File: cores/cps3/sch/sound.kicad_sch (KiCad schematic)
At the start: 68 parts, among them J1 AudioJack2, J2 AudioJack2, Q8 ZR

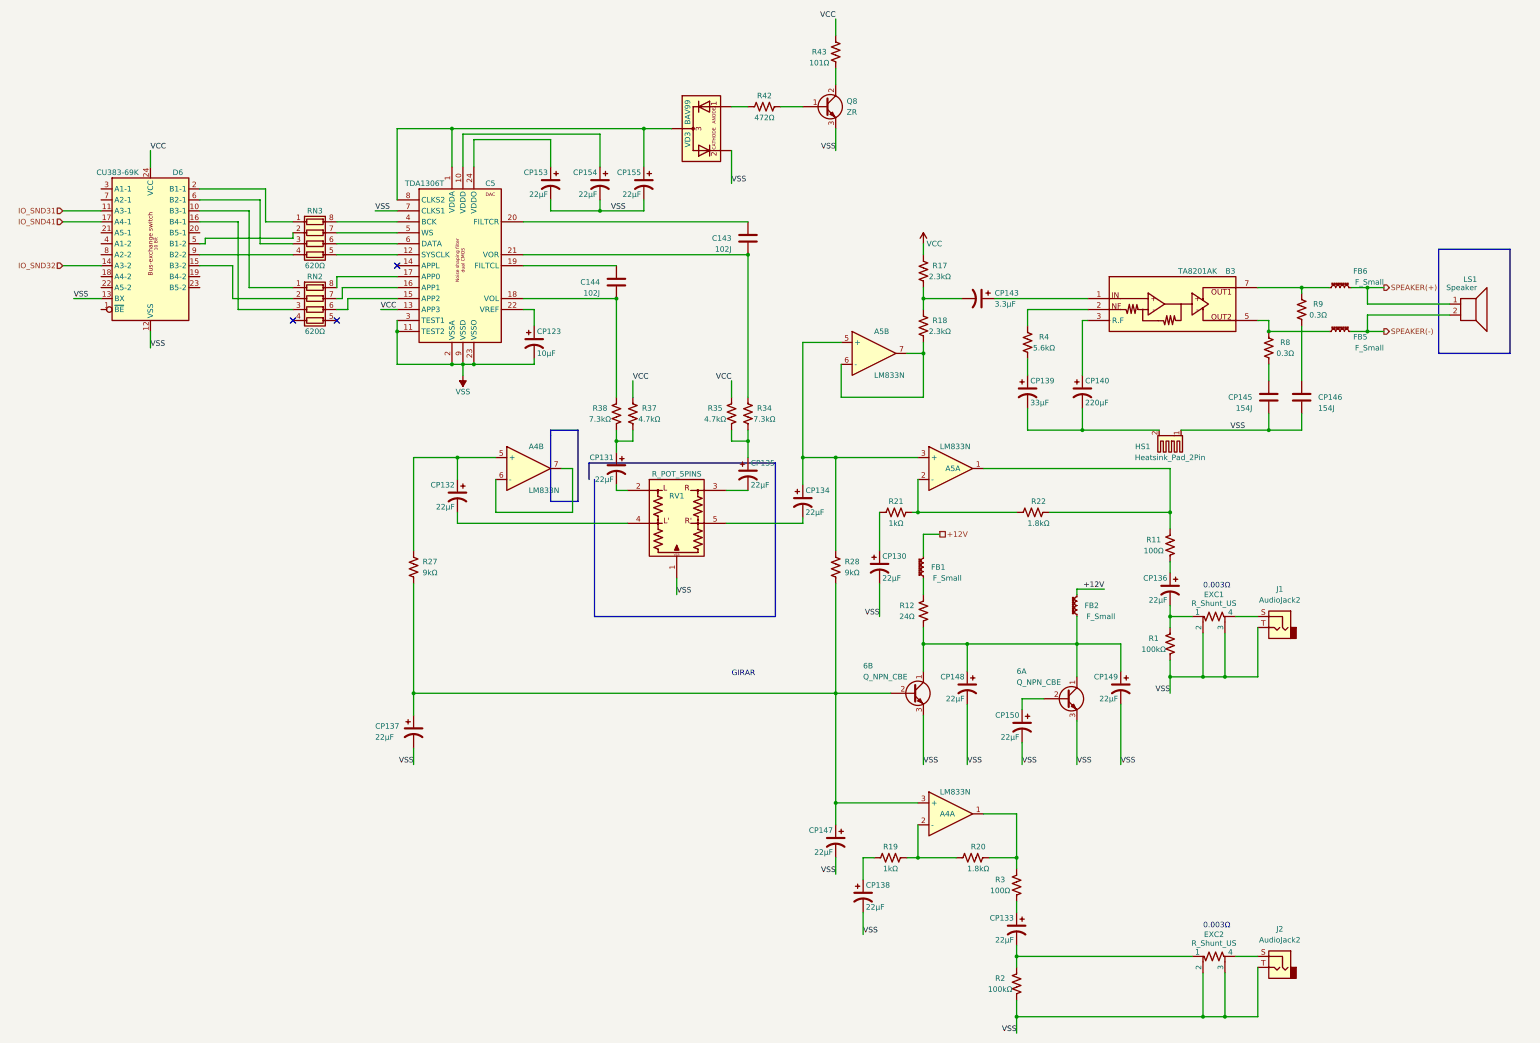
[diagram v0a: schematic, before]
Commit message: wip_cps3_vdac
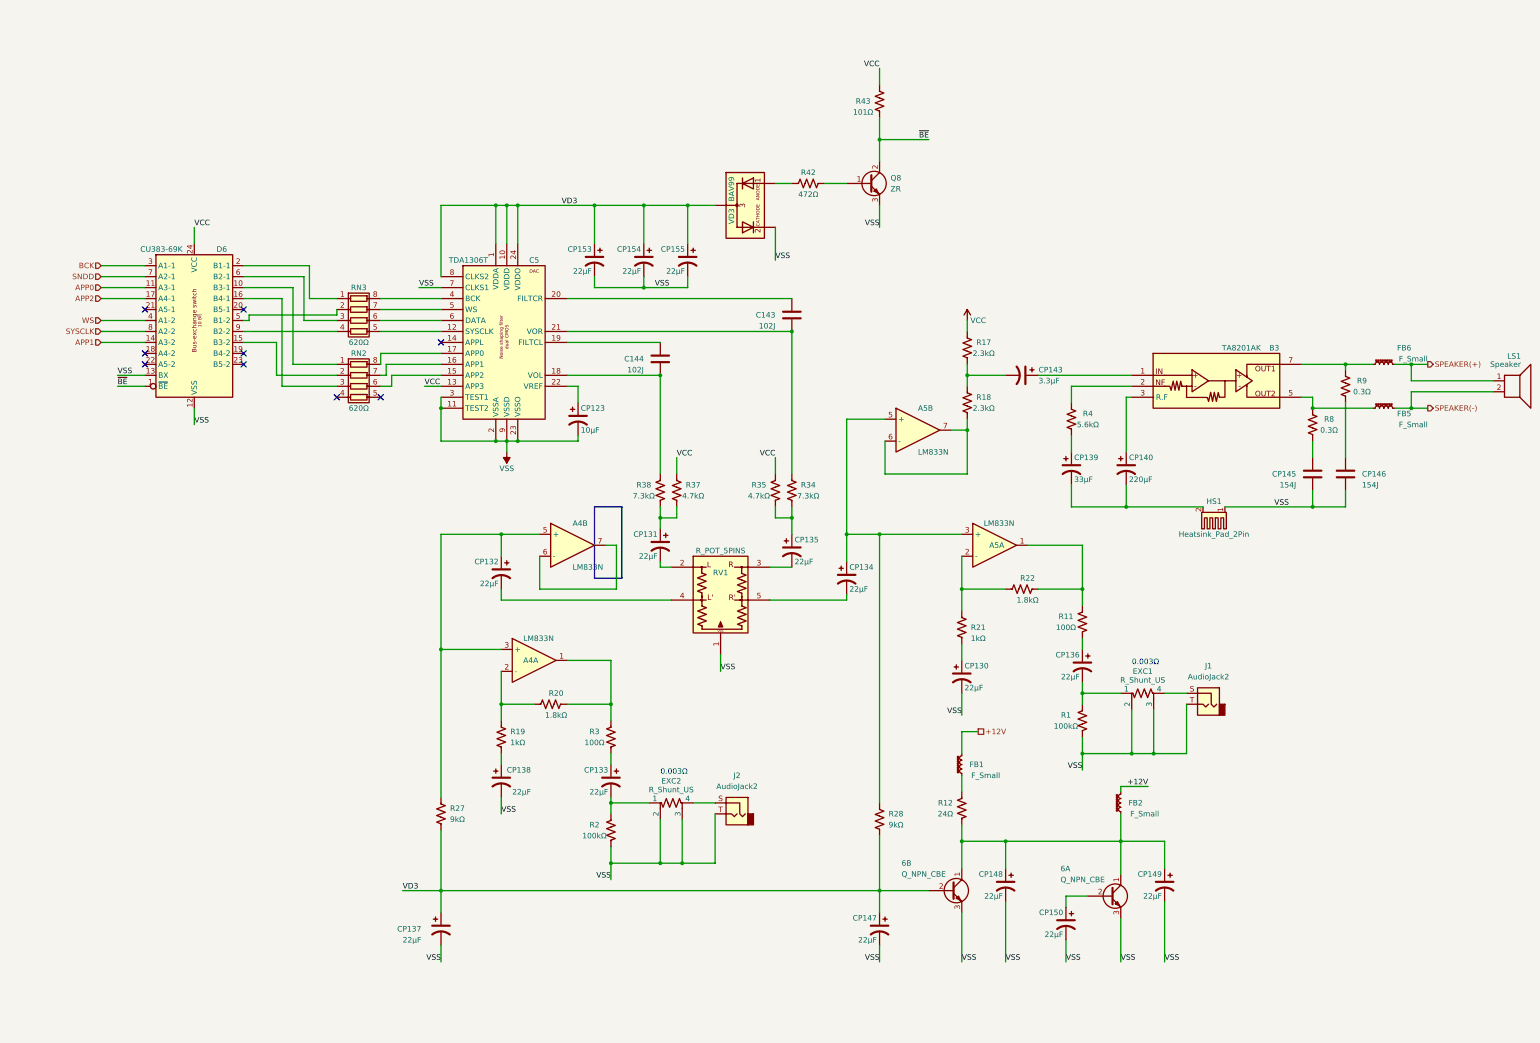
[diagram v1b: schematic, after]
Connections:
- net VD3: now reaches 6B.2 (B), CP137.1, CP147.1, R27.1, R28.1
- net VD3: now also C5.1 (VDDA), C5.10 (VDDD), C5.24 (VDDO), C5.8 (CLKS2), CP153.1, CP154.1, CP155.1, VD3.; no longer A4.3 (+)
- net at A4.5 (+), CP132.1, R27.2: now also A4.3 (+)
- net ~{BE}: now reaches D6.1 (~{BE})
- net ~{BE}: now also Q8.2 (C), R43.1
- net BCK: now reaches D6.3 (A1-1)
- net WS: now reaches D6.4 (A1-2)
- net SNDD: now reaches D6.7 (A2-1)
- net SYSCLK: now reaches D6.8 (A2-2)
- net IO_SND31 renamed APP0
- net IO_SND32 renamed APP1
- net IO_SND41 renamed APP2
- no-connect marks 3 -> 9
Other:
- note removed: "GIRAR"
- moved on the sheet: 6A, 6B, A4A, A4B, A5A, A5B, B3, C143, C144, C5, CP123, CP130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
